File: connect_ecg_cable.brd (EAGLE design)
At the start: 39.6 x 53.3 mm, 3 parts, among them J1 Conncector1, X1 Conncector2

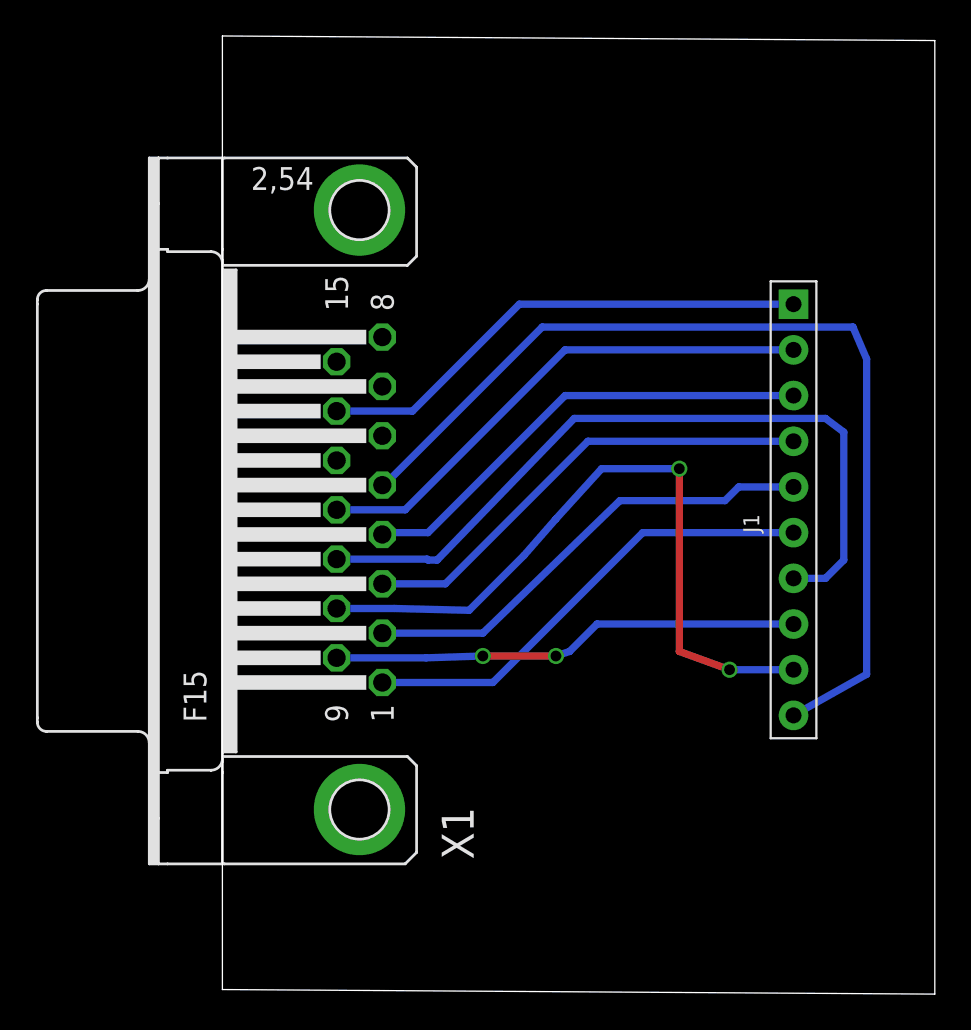
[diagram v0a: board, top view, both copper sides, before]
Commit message: did small size about connector
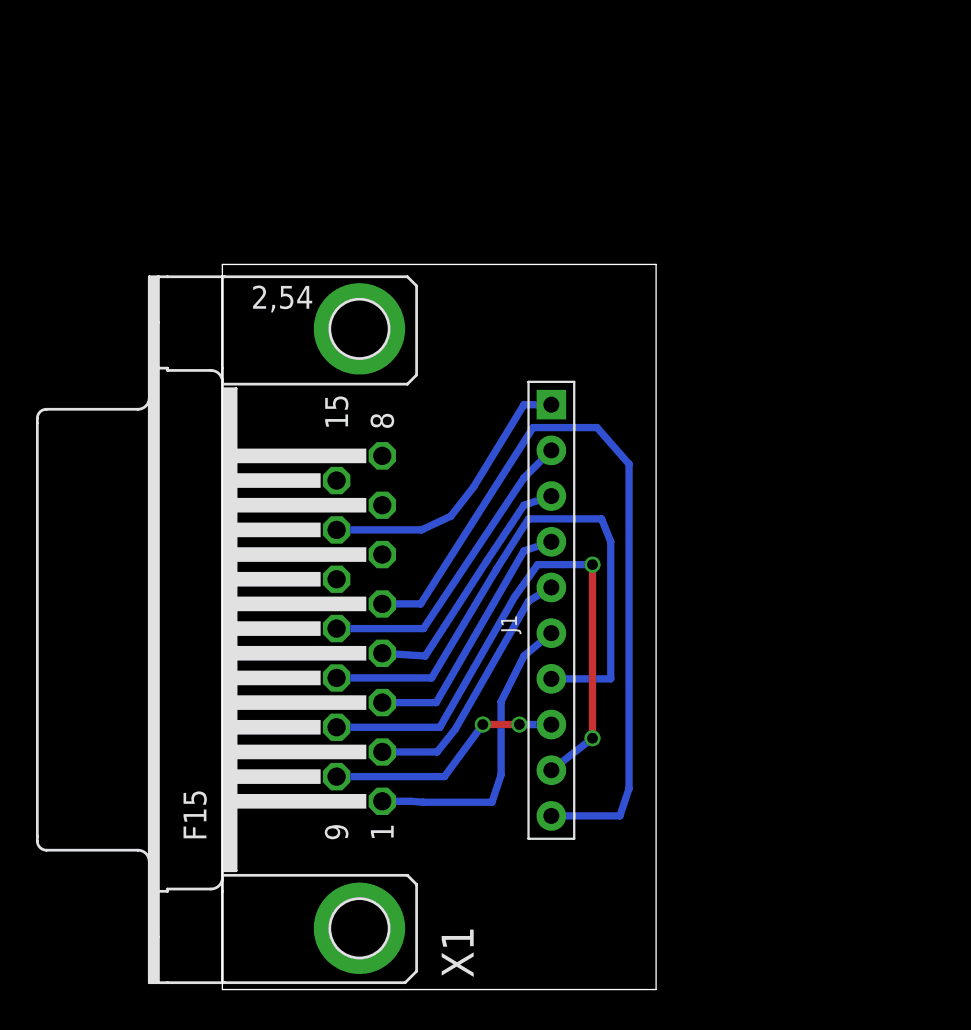
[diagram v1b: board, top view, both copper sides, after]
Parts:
- moved U$1 29.1 mm to (19.3, 1.02)
- moved J1 14.6 mm to (18.3, 21.1)
- moved X1 6.60 mm to (7.62, 20.1)
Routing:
- net RA: track 26.1 -> 13.4 mm
- net RL: track 27.9 -> 15.5 mm
- net V5: track 26.1 -> 14.0 mm
- net V1: track 29.1 -> 17.1 mm
- net V3: track 26.2 -> 14.3 mm
- net V4: track 26.1 -> 14.3 mm
- net V6: track 53.9 -> 43.5 mm
- net LL: track 42.1 -> 32.0 mm
- net V2: track 26.3 -> 16.6 mm
- net LA: track 39.2 -> 31.9 mm
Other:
- board size 39.6 x 53.3 mm -> 24.1 x 40.3 mm
